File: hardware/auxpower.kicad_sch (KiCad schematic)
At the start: 6 parts

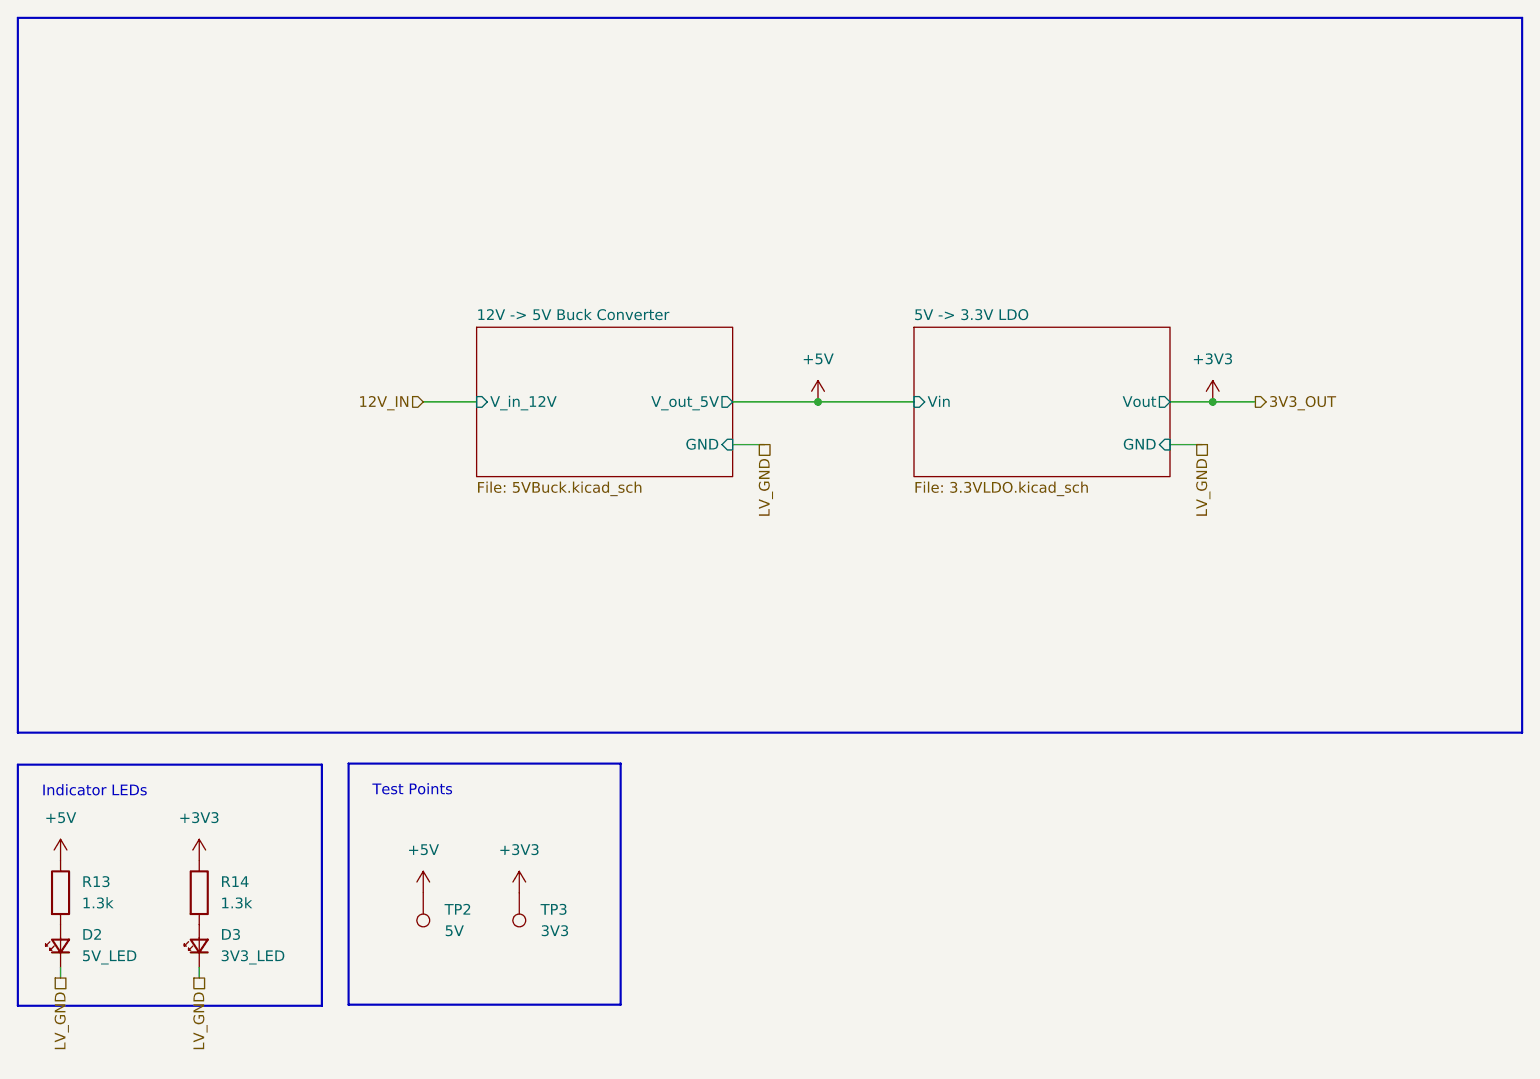
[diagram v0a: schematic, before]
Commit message: try smth on laptop
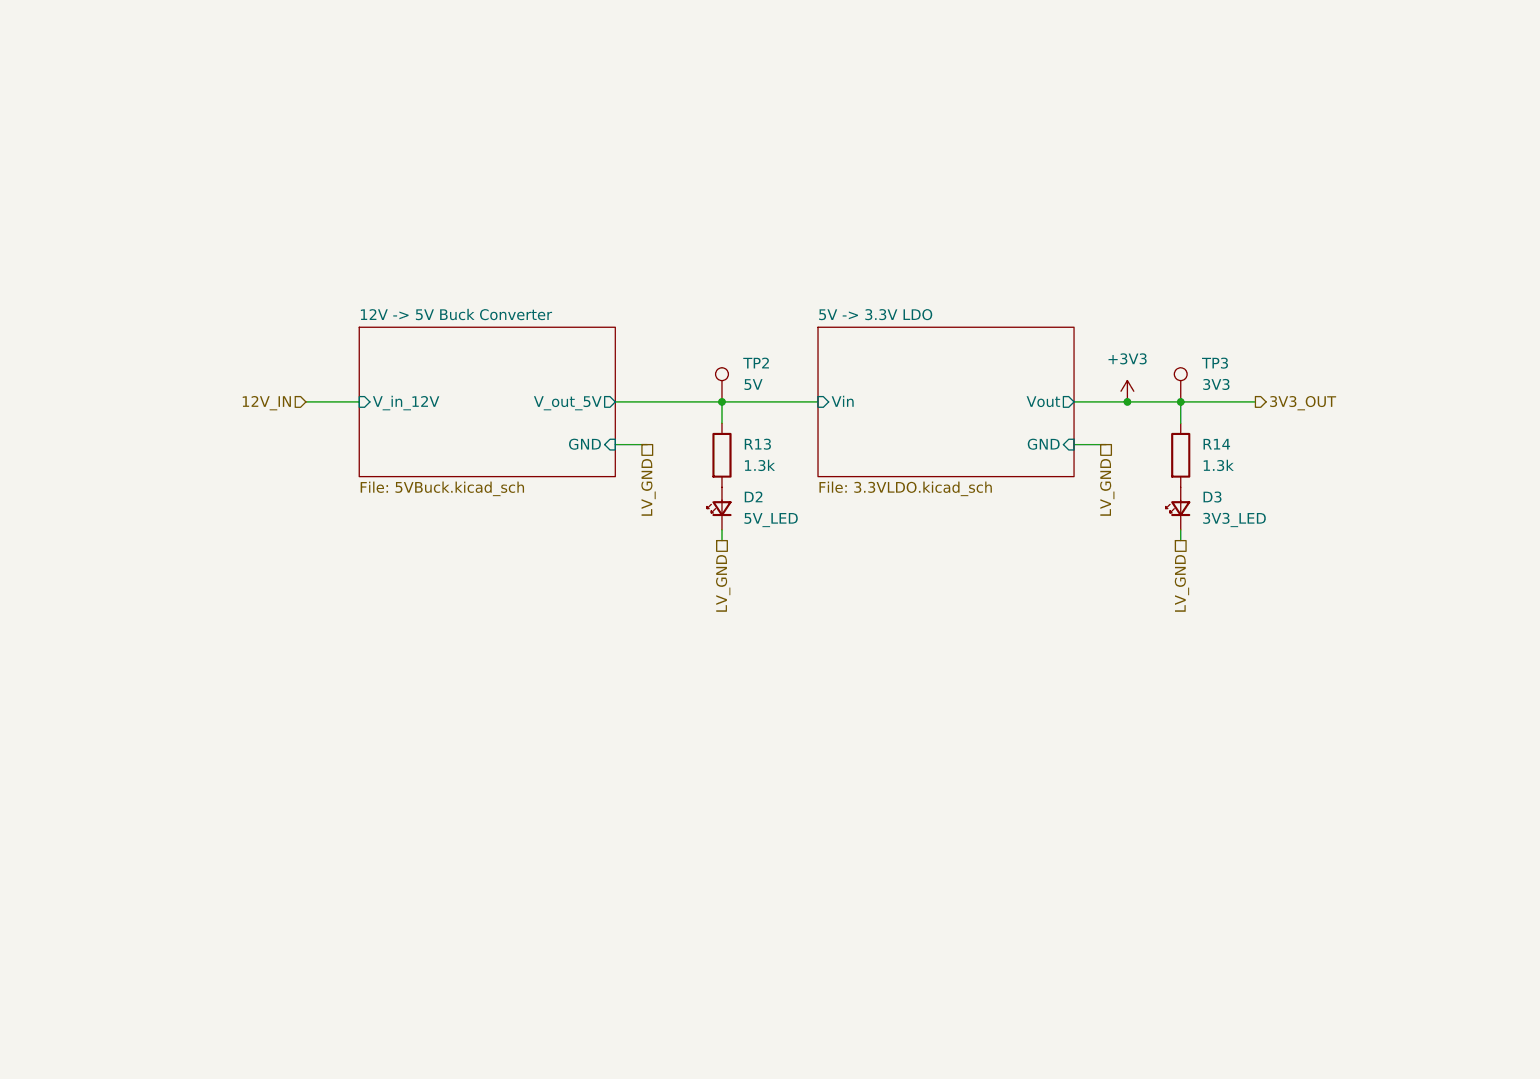
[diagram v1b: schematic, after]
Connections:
- net +5V renamed 12V -> 5V Buck Converter/V_out_5V
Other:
- note removed: "Indicator LEDs"
- note removed: "Test Points"
- moved on the sheet: D2, D3, R13, R14, TP2, TP3
